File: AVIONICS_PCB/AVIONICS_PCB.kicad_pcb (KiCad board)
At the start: 2 copper layers, 5 parts, among them U1 ESP32-S3-DevKitC

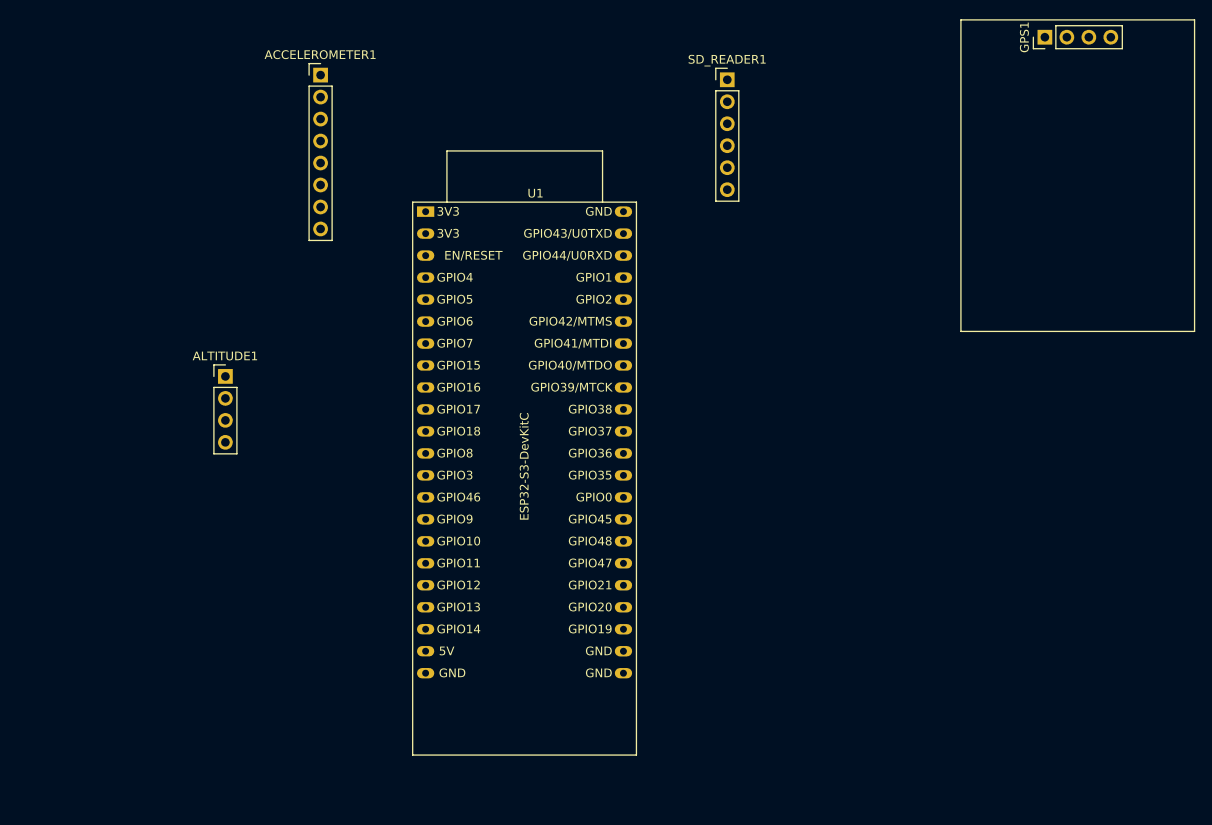
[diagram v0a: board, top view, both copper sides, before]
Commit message: Added power system
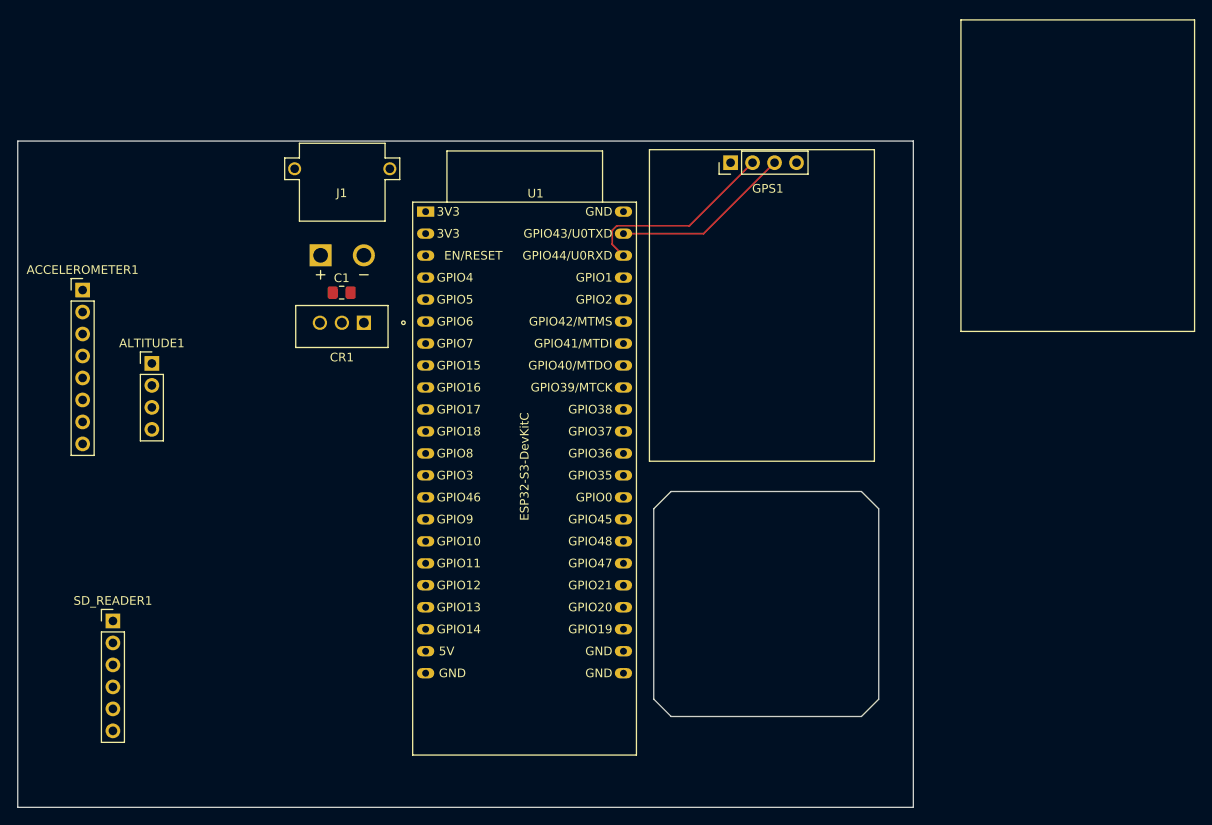
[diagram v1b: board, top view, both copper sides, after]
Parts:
- added C1: C, Capacitor_SMD:C_0805_2012Metric_Pad1.18x1.45mm_HandSolder, F.Cu at (128.9, 81.0)
- added CR1: LD1117V33, LD1117V33:TO-220_STM, F.Cu at (131.5, 84.5)
- added J1: XT30PW-M, XT30PW-M:AMASS_XT30PW-M, F.Cu at (129.0, 66.7)
- moved SD_READER1 94.6 mm to (102.5, 119.0)
- moved GPS1 39.1 mm to (173.9, 66.0)
- moved ACCELEROMETER1 37.1 mm to (99.0, 80.7)
- moved ALTITUDE1 8.63 mm to (107.0, 89.2)
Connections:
- U1 pad 42: RX -> TX
- U1 pad 43: TX -> RX
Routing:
- net TX: track 0.00 -> 22.9 mm
- net RX: track 0.00 -> 20.9 mm
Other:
- board outline added: 103.5 x 77 mm
